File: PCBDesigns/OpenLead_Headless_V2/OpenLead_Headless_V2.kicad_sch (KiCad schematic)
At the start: 40 parts, among them J1 Conn_01x01, J2 Conn_01x01, J3 Conn_01x07_Pin, J4 Battery, J5 Conn_01x01, J6 Conn_01x07_Pin, J7 Conn_01x02, J8 Conn_01x03_Pin, Q1 AO3400A MOSFET, Q2 AO3400A MOSFET, U1 LM4060 - 1.25V

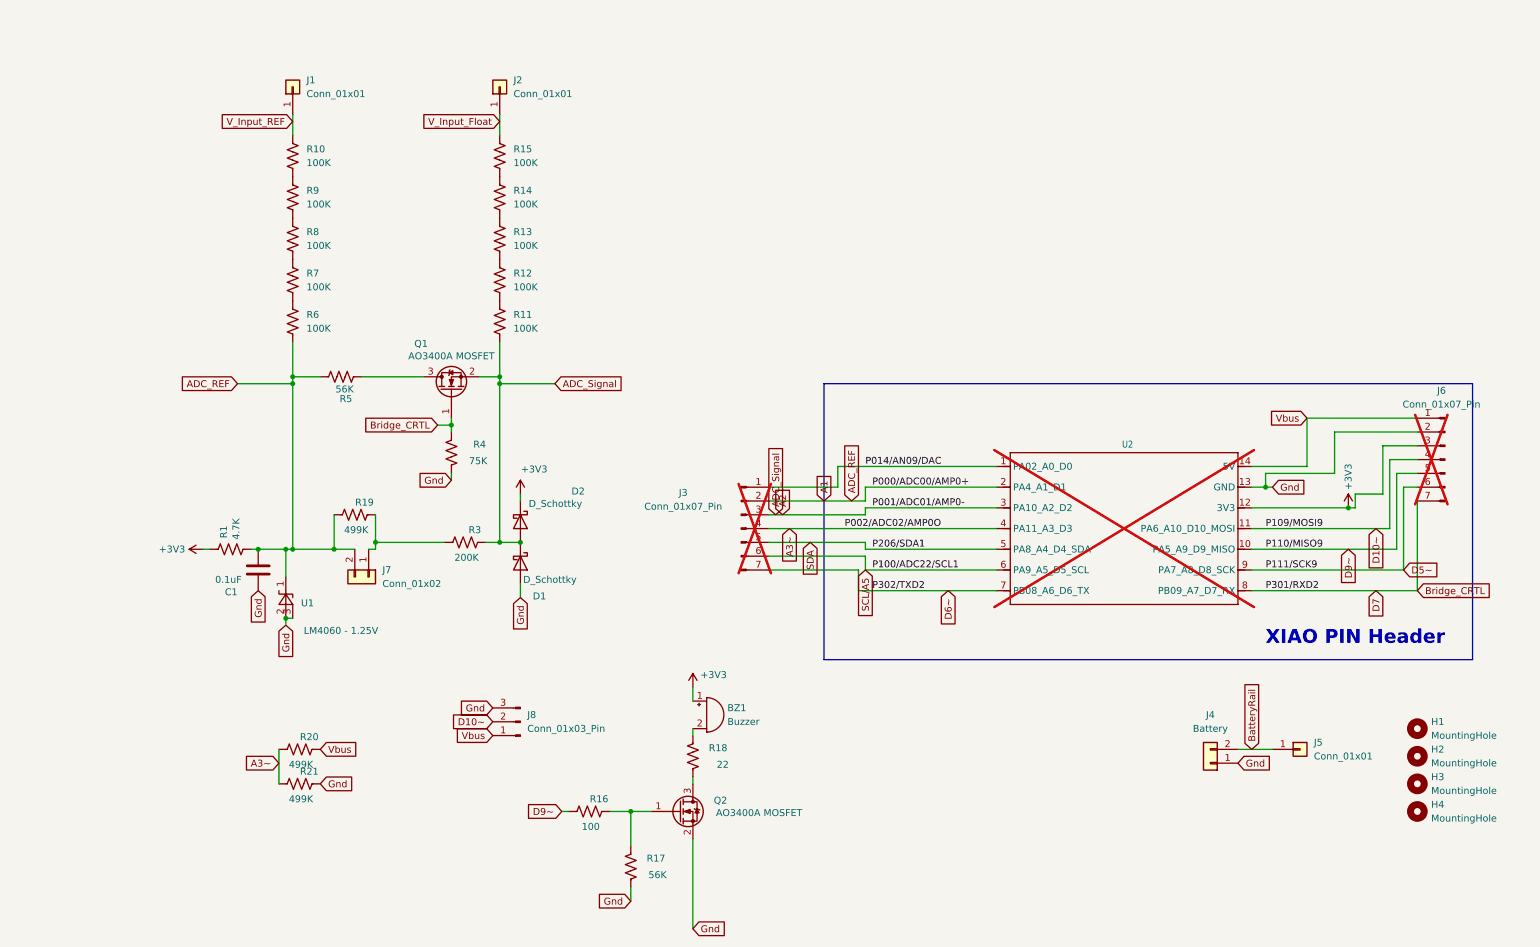
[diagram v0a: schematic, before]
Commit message: PCB design updates for Blinky Hawk
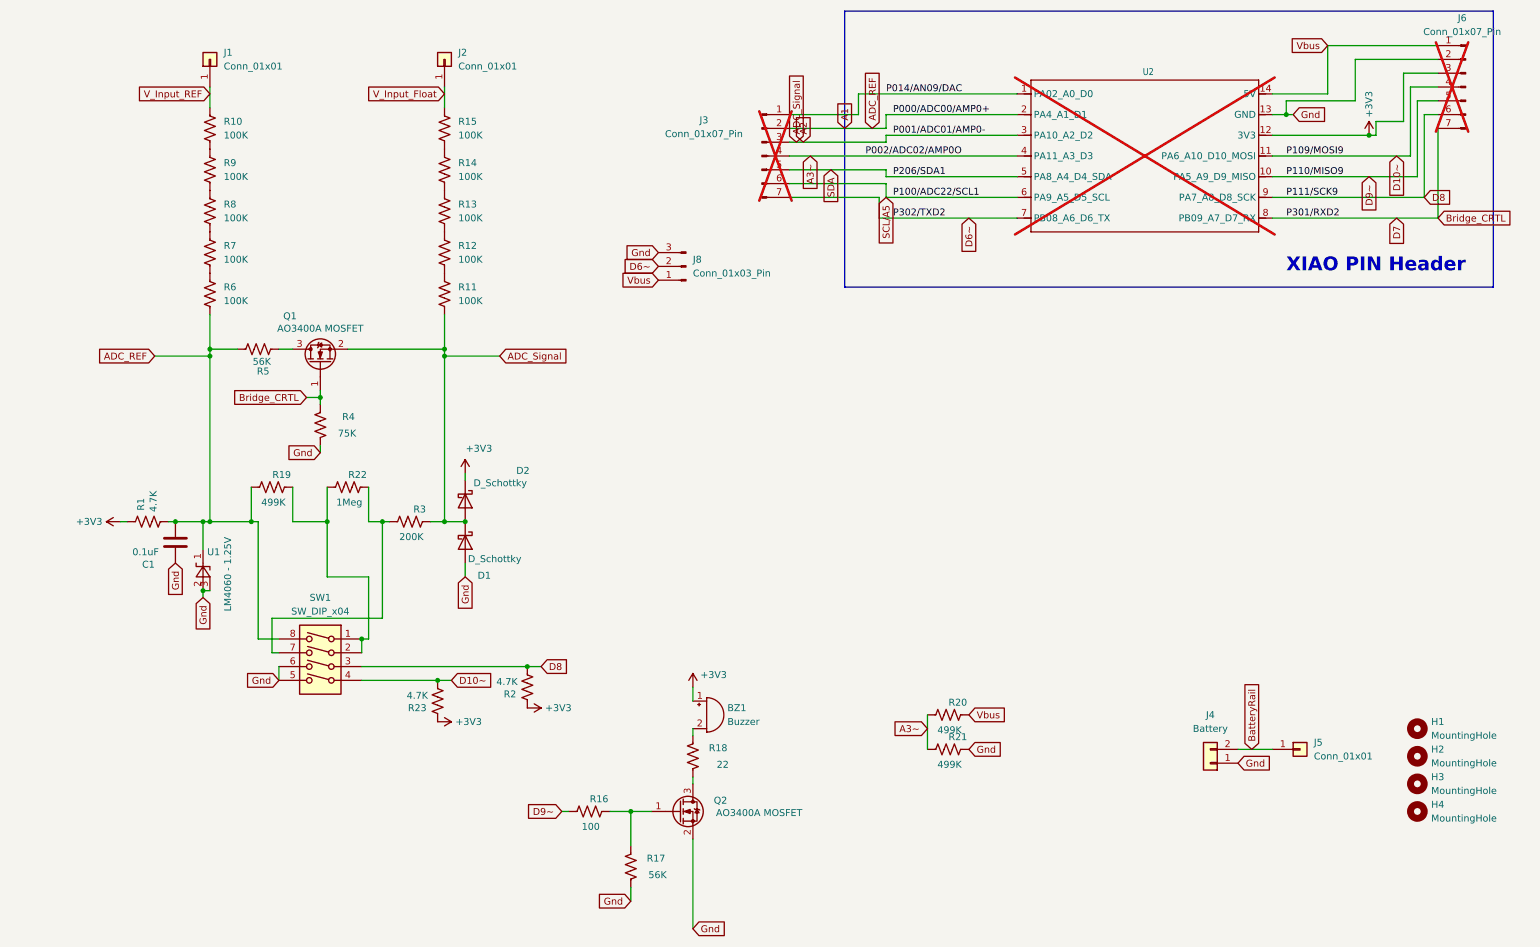
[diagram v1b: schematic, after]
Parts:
- removed J7: Conn_01x02, Connector_PinHeader_2.54mm:PinHeader_1x02_P2.54mm_Vertical, symbol Connector_Generic:Conn_01x02
- added R2, R23: 4.7K, Resistor_SMD:R_0805_2012Metric, symbol Device:R_US
- added R22: 1Meg, Resistor_SMD:R_0805_2012Metric, symbol Device:R_US
- added SW1: SW_DIP_x04, Button_Switch_SMD:SW_DIP_SPSTx04_Slide_KingTek_DSHP04TS_W7.62mm_P1.27mm, symbol Switch:SW_DIP_x04
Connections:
- net +3V3: now also R2.1, R23.1
- net A1: now also SW1.8
- net D10~: now also R23.2, SW1.4; no longer J8.2 (Pin_2)
- net D6~: now also J8.2 (Pin_2)
- net Gnd: now also SW1.5, SW1.6
- net at R19.2: now also R22.1, SW1.1, SW1.2; no longer R3.1
- net D5~ renamed D8
- net D8: now also R2.2, SW1.3
- new net: R22.2, R3.1, SW1.7
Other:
- moved on the sheet: C1, D1, D2, J1, J2, J3, J6, J8, Q1, R1, R10, R11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

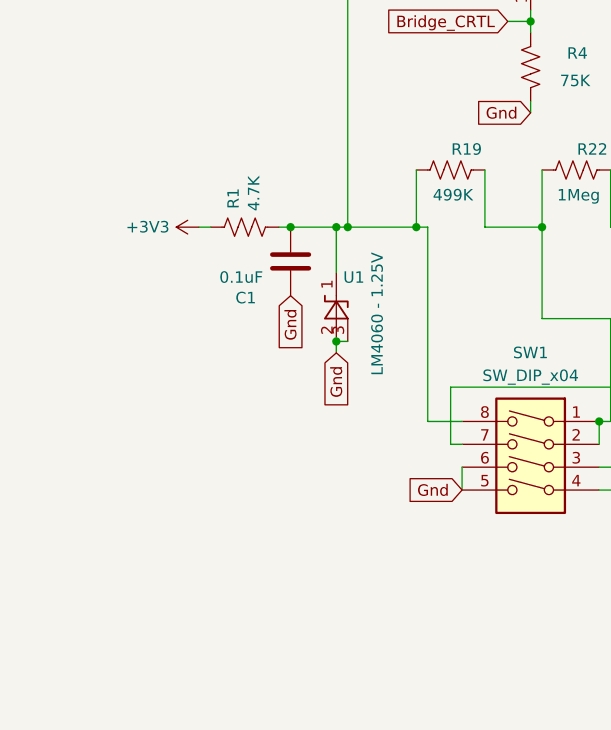
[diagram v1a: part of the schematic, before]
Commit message: PCB Design Updates
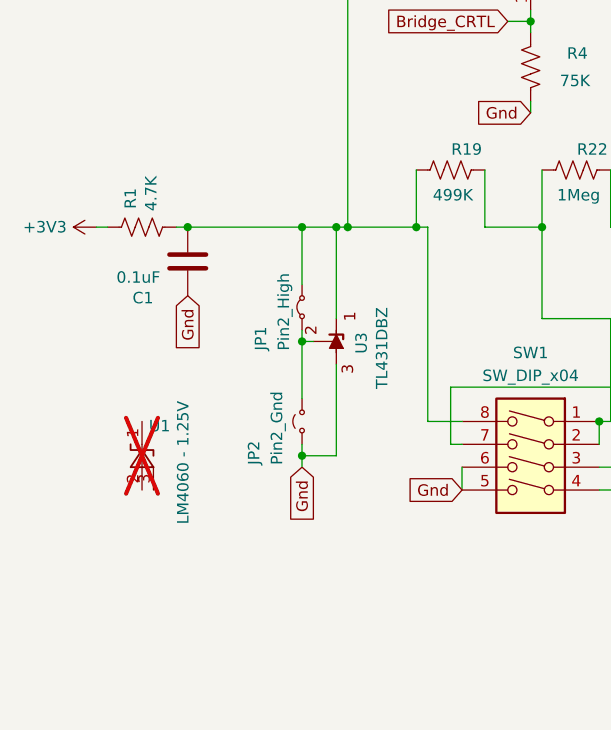
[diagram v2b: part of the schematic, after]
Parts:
- added JP1: Pin2_High, Jumper:SolderJumper-2_P1.3mm_Bridged_Pad1.0x1.5mm, symbol Jumper:Jumper_2_Small_Bridged
- added JP2: Pin2_Gnd, Jumper:SolderJumper-2_P1.3mm_Open_TrianglePad1.0x1.5mm, symbol Jumper:Jumper_2_Small_Open
- added U3: TL431DBZ, Package_TO_SOT_SMD:SOT-23, symbol Reference_Voltage:TL431DBZ
- BZ1: footprint Buzzer_Beeper:Buzzer_Murata_PKLCS1212E -> Buzzer_Beeper:Buzzer_12x9.5RM7.6
- U1: now not fitted
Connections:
- net A1: now also JP1.2 (B), U3.1 (K); no longer U1.1 (K)
- net Gnd: now also JP2.1 (A), U3.3 (A); no longer U1.2 (A), U1.3 (nc_(gnd))
- new net: JP1.1 (A), JP2.2 (B), U3.2 (REF)
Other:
- moved on the sheet: C1, R1
